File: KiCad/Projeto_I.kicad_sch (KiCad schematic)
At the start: 41 parts, among them J1 PORTA, J2 PORTB, J3 PORTC, J4 USB_B_Micro, J5 Barrel_Jack_Switch, Q1 PMOS, SW1 reset, U1 PIC18F4550-IP, U2 LM7805, U3 LM358, U4 AMS1117, Y1 16MHz

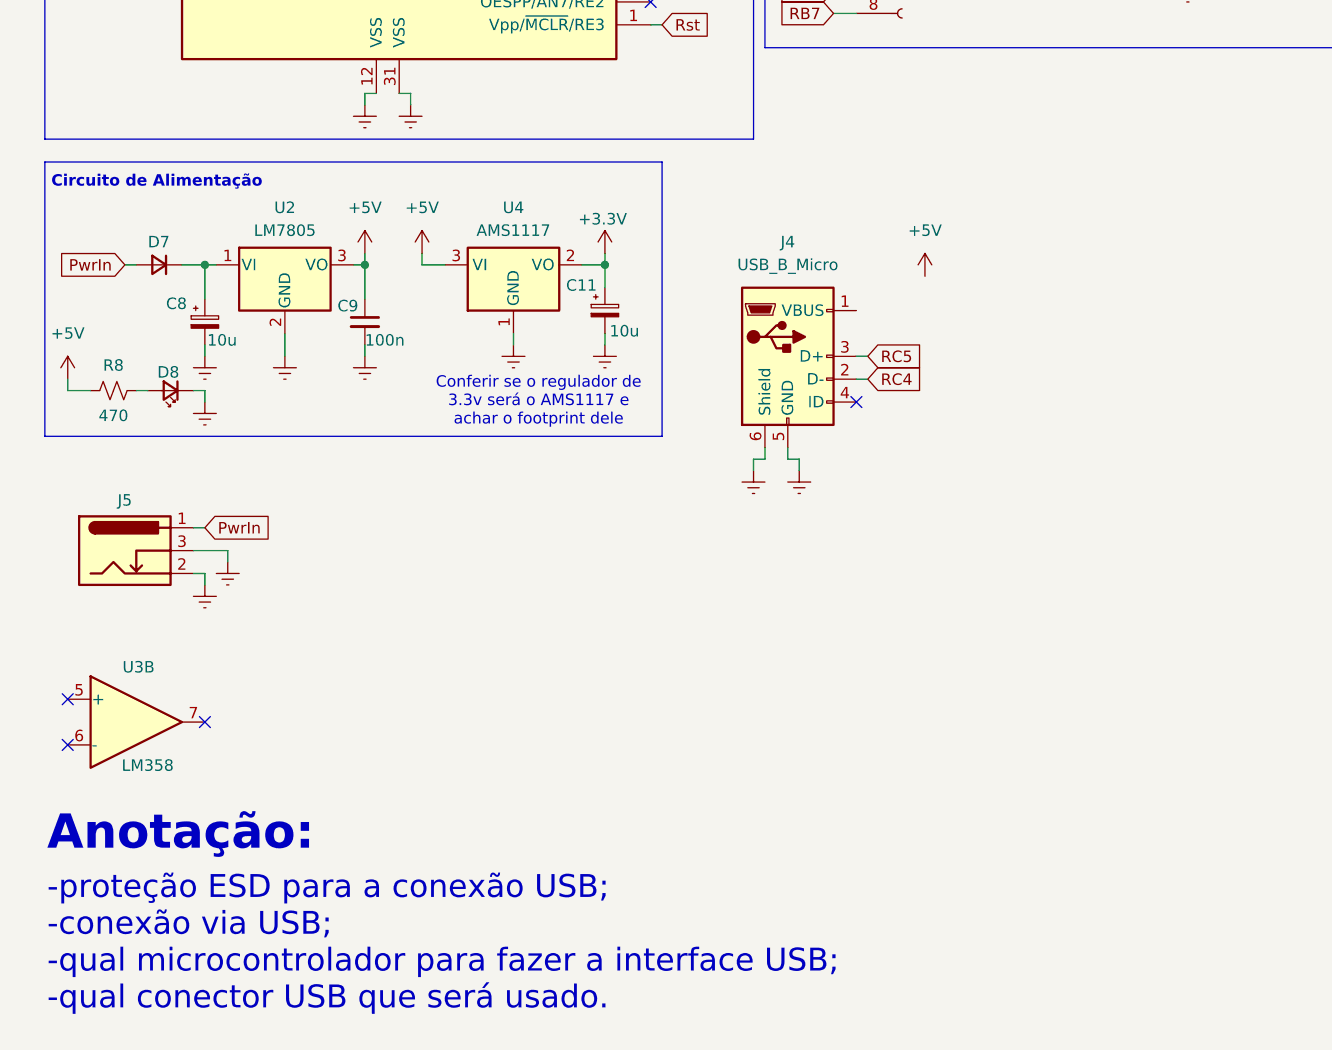
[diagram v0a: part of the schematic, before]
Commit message: AUla do dia 04/04/2025
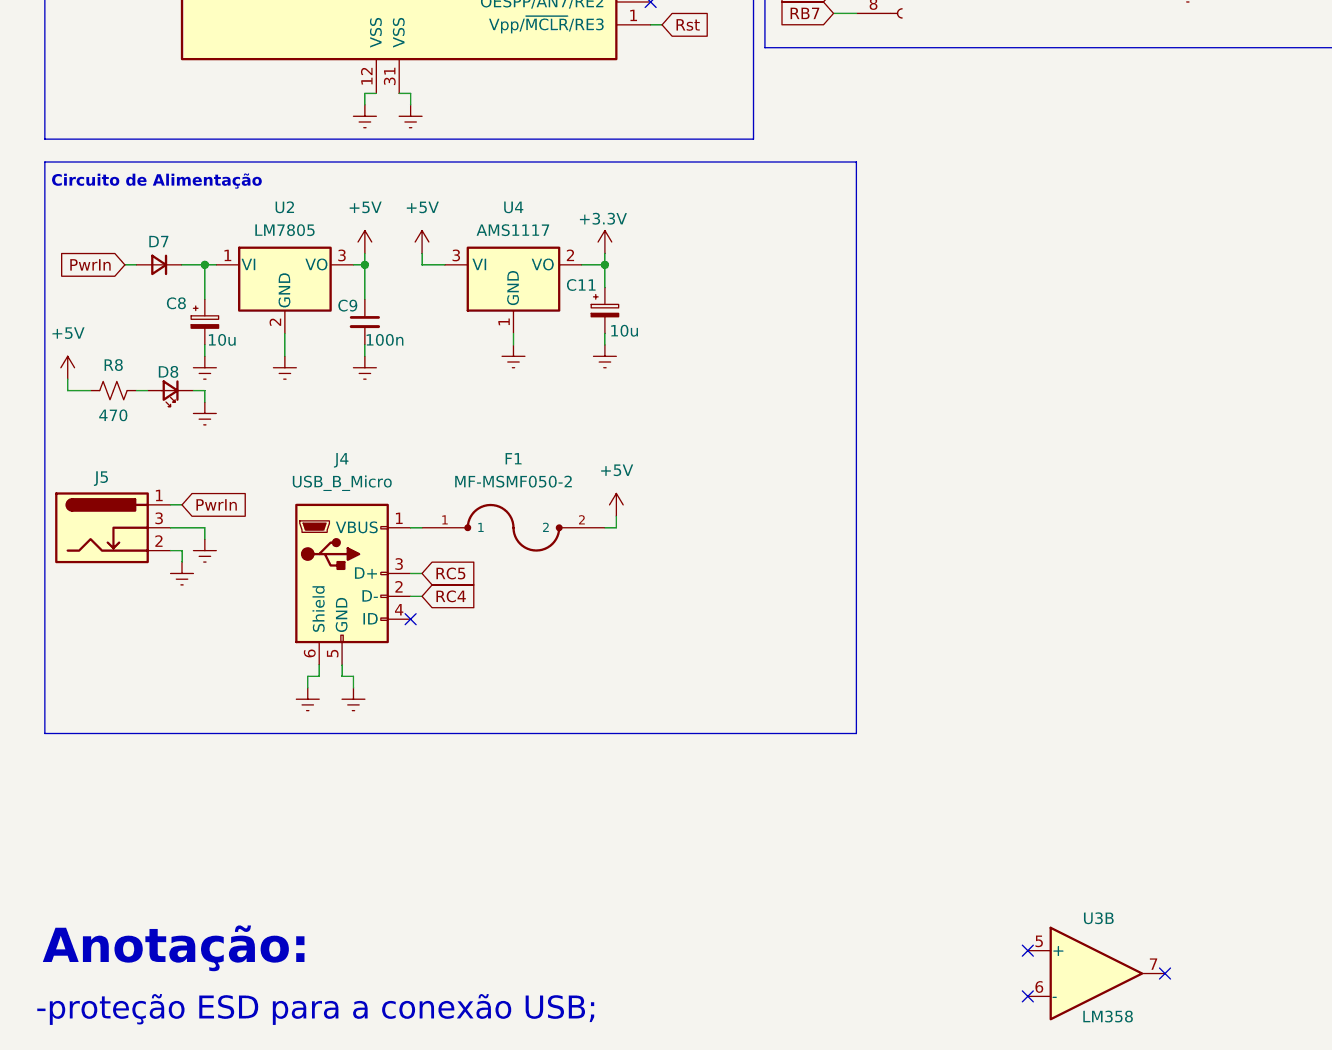
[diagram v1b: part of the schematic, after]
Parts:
- added F1: MF-MSMF050-2, Library:FUSM4632X85, symbol MF-MSMF050-2:MF-MSMF050-2
- C1: footprint Capacitor_THT:C_Disc_D7.5mm_W5.0mm_P7.50mm -> Capacitor_THT:C_Rect_L7.0mm_W2.5mm_P5.00mm
- C11, C8: footprint (none) -> Capacitor_THT:CP_Radial_D10.0mm_P3.80mm
- C2: footprint (none) -> Capacitor_THT:C_Rect_L7.0mm_W2.5mm_P5.00mm
- Q1: footprint (none) -> Package_TO_SOT_THT:TO-92L_HandSolder
- U4: footprint (none) -> Package_TO_SOT_SMD:SOT-223-3_TabPin2
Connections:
- net +5V: now also F1.2
- net at J4.1 (VBUS): now also F1.1
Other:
- note added: "-proteção ESD para a conexão USB;"
- note removed: "-proteção ESD para a conexão USB; -conexão via USB; -qual microcontrolador para fazer a interface USB; -qual conector USB que será usado."
- note removed: "Conferir se o regulador de 3.3v será o AMS1117 e achar o footprint dele"
- moved on the sheet: J4, J5, U3B
